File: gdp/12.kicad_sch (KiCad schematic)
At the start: 19 parts, among them IC1 74LS74, IC12 PAL16R4, IC51 74LS14, IC64 74LS123, IC66 74S00, IC71 74LS04

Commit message: Fixes footprints R34 R27
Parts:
- R27: footprint GDP:R_XL -> GDP:R_XL_narrow
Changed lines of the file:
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@@
 			)
 		)
-		(property "Footprint" "GDP:R_XL"
+		(property "Footprint" "GDP:R_XL_narrow"
 			(at 142.24 43.942 90)
 			(effects

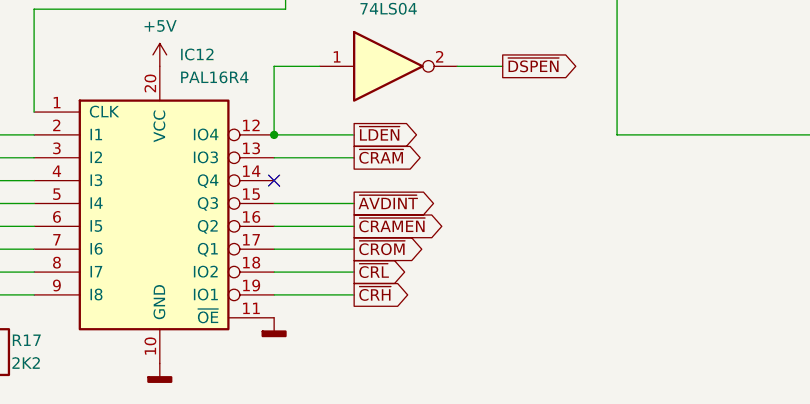
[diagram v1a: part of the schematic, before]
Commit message: Fixes resistor footprints
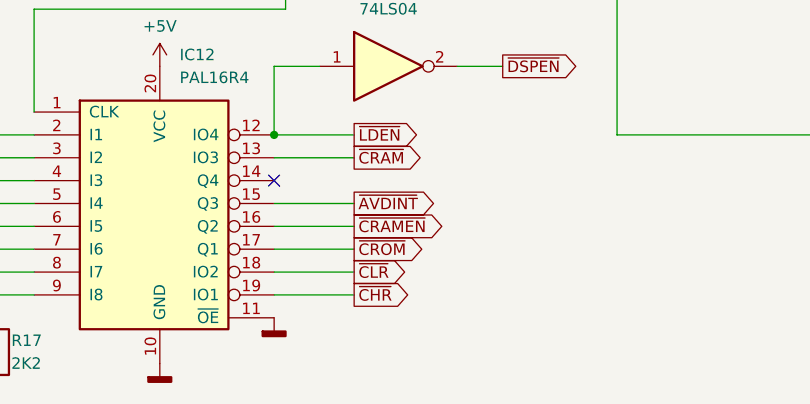
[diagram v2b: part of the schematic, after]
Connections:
- net ~{CRH} renamed ~{CHR}
- net ~{CRL} renamed ~{CLR}
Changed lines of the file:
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@@
 		)
 	)
-	(global_label "~{CRH}"
+	(global_label "~{CHR}"
 		(shape output)
 		(at 133.35 158.75 0)
@@
 		)
 	)
-	(global_label "~{CRL}"
+	(global_label "~{CLR}"
 		(shape output)
 		(at 133.35 156.21 0)
